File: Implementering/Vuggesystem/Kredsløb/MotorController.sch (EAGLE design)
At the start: 31 parts, among them IC1 74HC08N, IC2 74HC04N

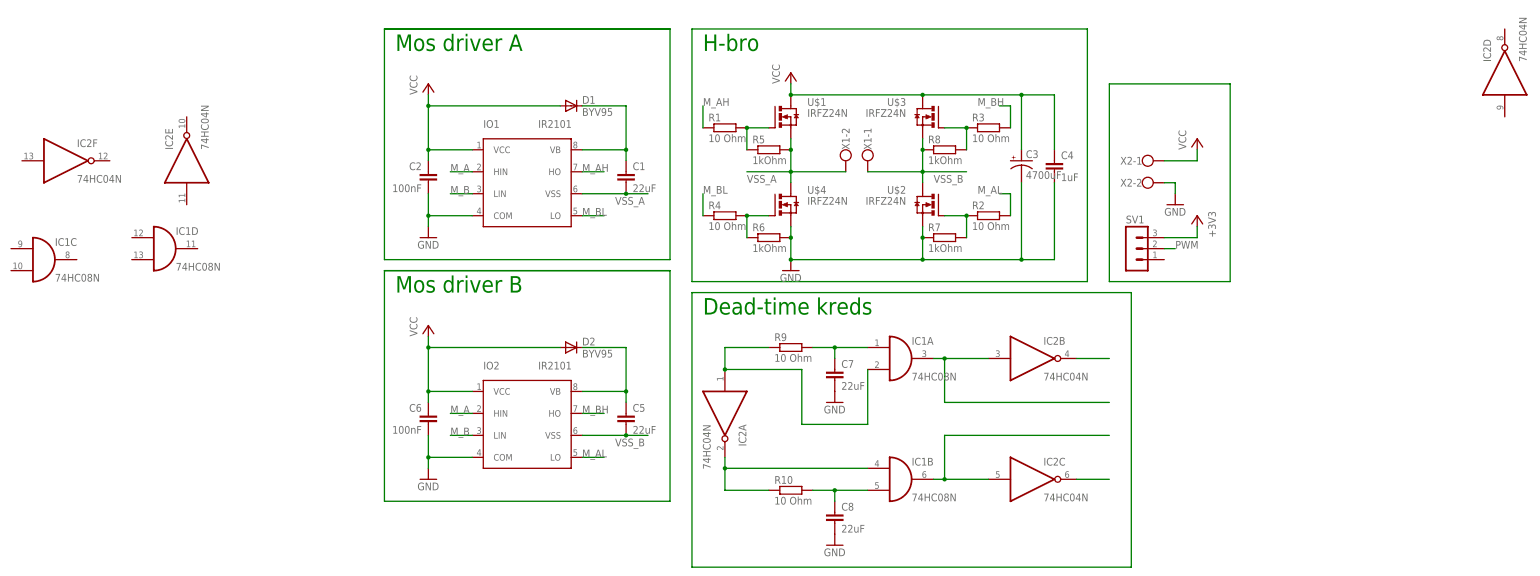
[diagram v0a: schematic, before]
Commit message: felix
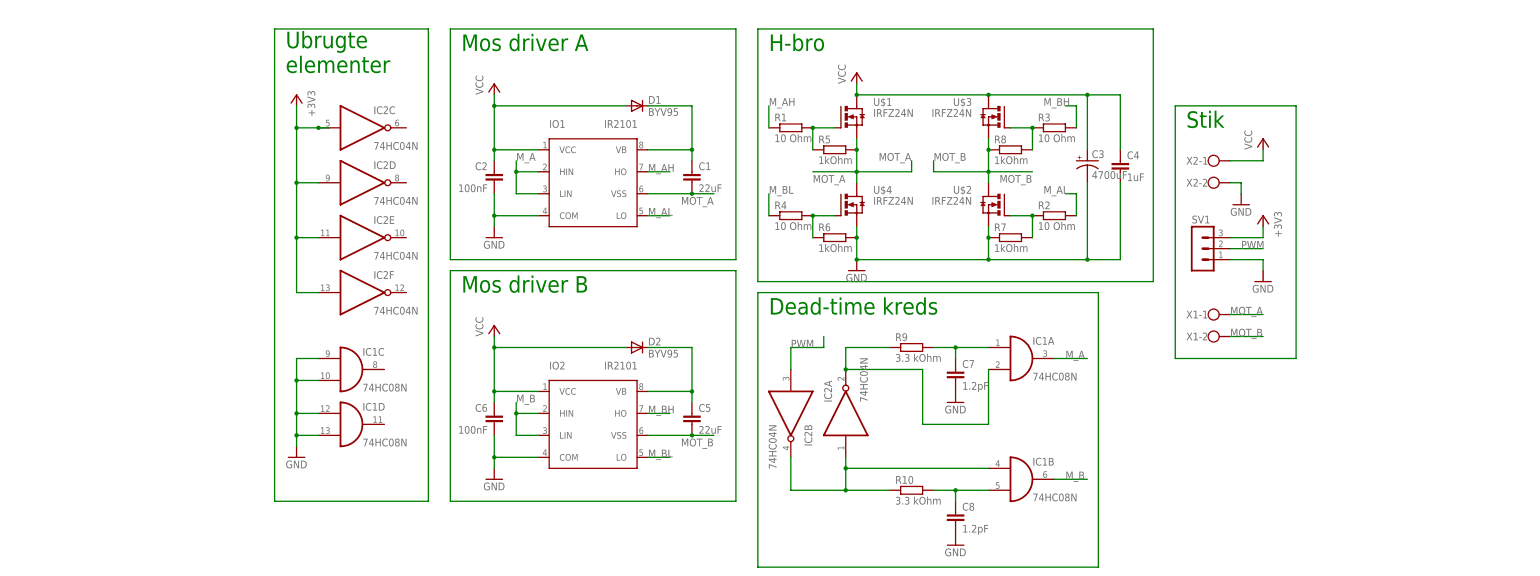
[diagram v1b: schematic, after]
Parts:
- C7, C8: value 22uF -> 1.2pF
- R10, R9: value 10 Ohm -> 3.3 kOhm
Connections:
- removed net N$11: IC1B.O, IC2C.I
- removed net N$14: IC1A.I1, IC2A.I, R9.1
- removed net N$17: IC2B.O
- removed net N$18: IC2C.O
- removed net N$19: IC1B.I0, IC2A.O, R10.1
- removed net VSS_A: C1.2, IO1.VSS, R5.2, U$1.S, U$4.D, X1-2.KL
- removed net VSS_B: C5.2, IO2.VSS, R8.1, U$2.D, U$3.S, X1-1.KL
- new net MOT_A: C1.2, IO1.VSS, R5.2, U$1.S, U$4.D, X1-1.KL
- new net MOT_B: C5.2, IO2.VSS, R8.1, U$2.D, U$3.S, X1-2.KL
- net +3V3: now also IC2C.I, IC2D.I, IC2E.I, IC2F.I
- net GND: now also IC1C.I0, IC1C.I1, IC1D.I0, IC1D.I1, SV1.1
- net M_A: now also IC1A.O, IO1.LIN; no longer IO2.HIN
- net M_AL: now also IO1.LO; no longer IO2.LO
- net M_B: now also IC1B.O, IO2.HIN; no longer IO1.LIN
- net M_BL: now also IO2.LO; no longer IO1.LO
- net N$10: now also IC1B.I0, IC2A.I, IC2B.O, R10.1; no longer IC1A.O, IC2B.I
- net PWM: now also IC1A.I1, IC2A.O, IC2B.I, R9.1
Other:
- note added: "Stik"
- note added: "Ubrugte elementer"
- moved on the sheet: C1, C2, C3, C4, C5, C6, C7, C8, D1, D2, IC1A, IC1B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

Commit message: har lavet print til motor kreds, og lavet lidt på motor kontrol -Felix
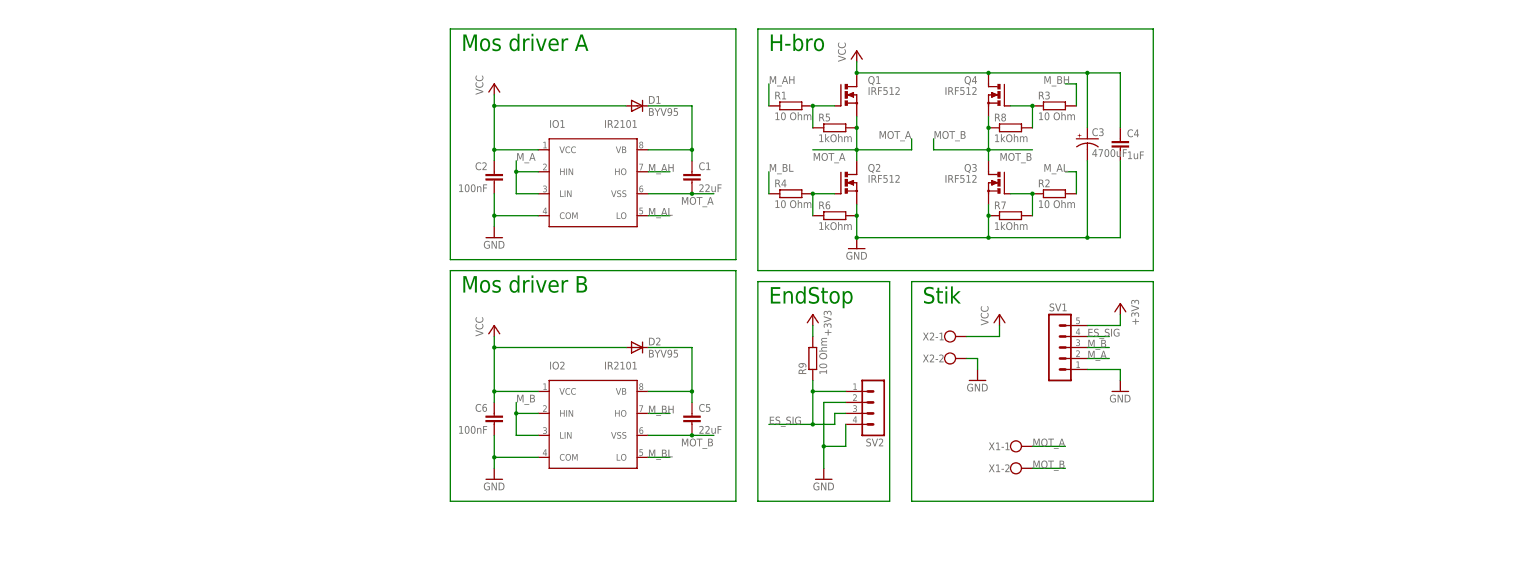
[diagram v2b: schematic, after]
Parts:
- removed C7, C8: 1.2pF, SparkFun-Passives:CAPPTH1
- removed IC1: 74HC08N, 74xx-eu:74HC08N
- removed IC2: 74HC04N, 74xx-eu:74HC04N
- removed R10: 3.3 kOhm, rcl:R-EU_0207/10
- removed U$1, U$2, U$3, U$4: IRFZ24N, transistor-power:IRFZ24N
- added Q1, Q2, Q3, Q4: IRF512, transistor-power:IRF512
- added SV2: (no value), con-lstb:MA04-1
- R9: value 3.3 kOhm -> 10 Ohm
- SV1: device con-lstb:MA03-1 -> con-lstb:MA05-1
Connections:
- removed net N$10: IC1B.I0, IC2A.I, IC2B.O, R10.1
- removed net N$15: C7.1, IC1A.I0, R9.2
- removed net N$16: C8.1, IC1B.I1, R10.2
- removed net PWM: IC1A.I1, IC2A.O, IC2B.I, R9.1, SV1.2
- new net ES_SIG: R9.1, SV1.4, SV2.1, SV2.3
- net +3V3: now also R9.2, SV1.5; no longer IC2C.I, IC2D.I, IC2E.I, IC2F.I, SV1.3
- net GND: now also Q2.S, Q3.S, SV2.2, SV2.4; no longer C7.2, C8.2, IC1C.I0, IC1C.I1, IC1D.I0, IC1D.I1, U$2.S, U$4.S
- net MOT_A: now also Q1.S, Q2.D; no longer U$1.S, U$4.D
- net MOT_B: now also Q3.D, Q4.S; no longer U$2.D, U$3.S
- net M_A: now also SV1.2; no longer IC1A.O
- net M_B: now also SV1.3; no longer IC1B.O
- net N$3: now also Q1.G; no longer U$1.G
- net N$4: now also Q2.G; no longer U$4.G
- net N$5: now also Q4.G; no longer U$3.G
- net N$6: now also Q3.G; no longer U$2.G
- net VCC: now also Q1.D, Q4.D; no longer U$1.D, U$3.D
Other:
- note added: "EndStop"
- note removed: "Dead-time kreds"
- note removed: "Ubrugte elementer"
- moved on the sheet: C3, C4, R1, R2, R3, R4, R5, R6, R7, R8, R9, X1-1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
